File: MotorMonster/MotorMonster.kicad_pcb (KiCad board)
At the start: 4 copper layers, 100 x 100 mm, 83 parts, among them J1 USB C Connector, J3 HV In, SW1 Boot, U1 XC6206, U2 USBLC6-2SC6, U3 RP2040, U4 W25Q128JVS, U5 LM5164DDA, Y1 12MHz

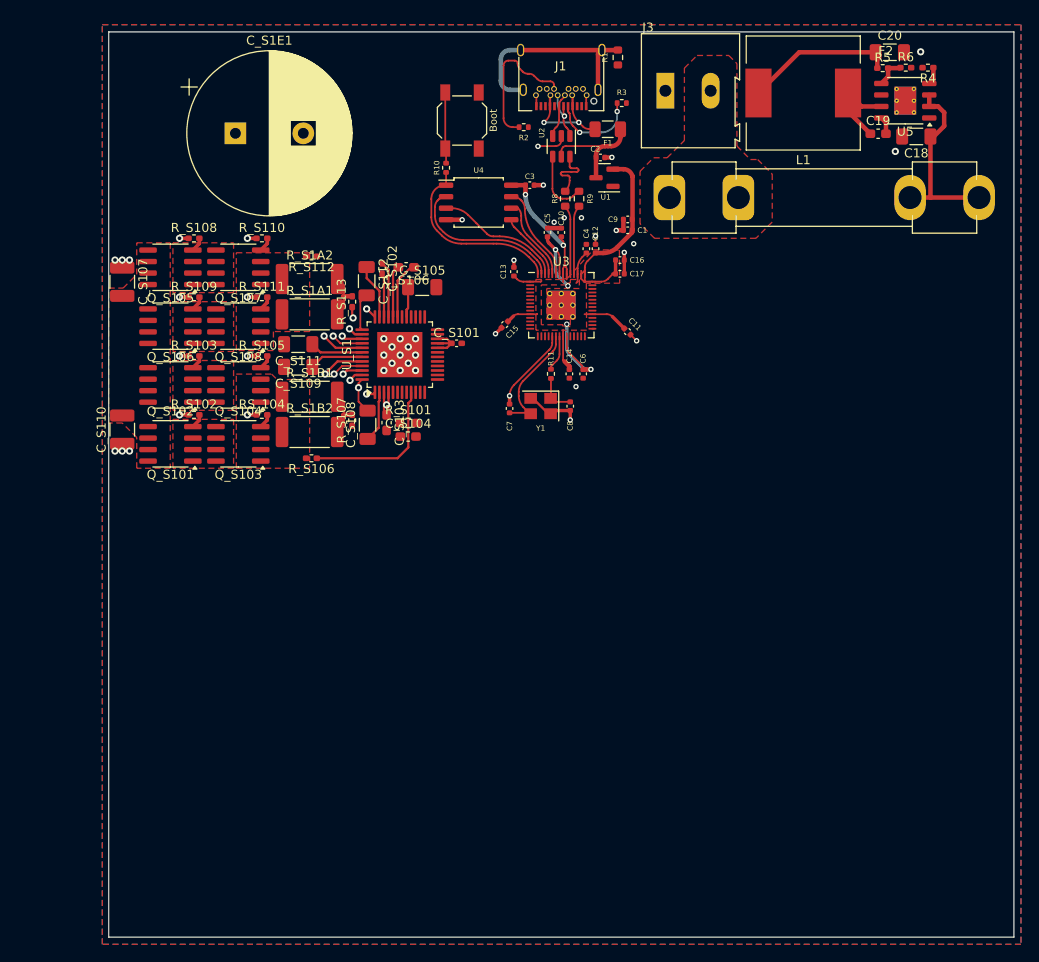
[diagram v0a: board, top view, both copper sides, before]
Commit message: fully laid out
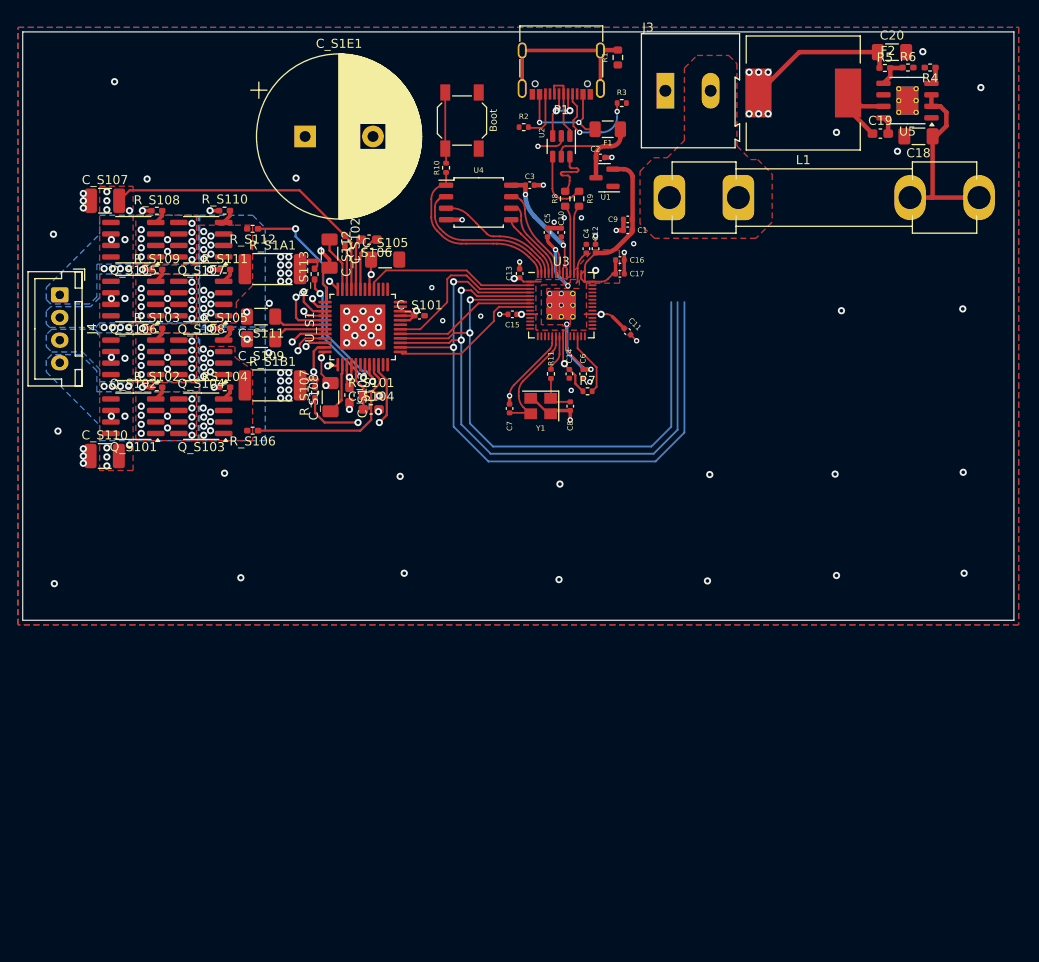
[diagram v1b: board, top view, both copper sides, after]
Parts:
- removed J1: USB C Connector, footprints:TYPE-C_24P_QCHT
- removed R_S1A2, R_S1B2: R, Resistor_SMD:R_2512_6332Metric_Pad1.40x3.35mm_HandSolder
- added J4: Conn_01x04, Connector_JST:JST_XH_B4B-XH-A_1x04_P2.50mm_Vertical, F.Cu at (84.6, 49.0)
- added P1: USB_C_Plug_USB2.0, Connector_USB:USB_C_Receptacle_G-Switch_GT-USB-7010ASV, F.Cu at (140.0, 23.1)
- added R7: 10k, Resistor_SMD:R_0402_1005Metric, F.Cu at (142.9, 59.7)
- moved C_S107 9.15 mm to (89.6, 38.6), turned to 0 degrees
- moved C_S1E1 7.71 mm to (111.7, 31.6)
- moved R_S112 7.18 mm to (105.9, 41.8)
- moved R_S106 7.18 mm to (105.9, 64.0)
- moved R_S1A1 6.47 mm to (108.1, 46.2)
- moved NT1 5.52 mm to (112.5, 58.4)
- moved NT2 5.48 mm to (112.5, 45.3)
- moved R_S113 5.15 mm to (112.8, 46.8)
- moved R_S110 5.14 mm to (102.8, 39.8)
- moved C_S105 5.11 mm to (120.5, 45.1)
- moved Q_S105 5.11 mm to (92.7, 43.0)
- moved Q_S106 5.11 mm to (92.7, 49.5)
- moved Q_S107 5.11 mm to (100.2, 43.0)
- moved Q_S108 5.11 mm to (100.2, 49.5)
- moved C_S101 5.11 mm to (124.3, 51.4)
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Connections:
- U3 pad 2: unconnected-(U3-GPIO0-Pad2) -> S1En
- U3 pad 3: unconnected-(U3-GPIO1-Pad3) -> S1Dir
- U3 pad 7: S1CS -> S1Step
- U3 pad 8: unconnected-(U3-GPIO6-Pad8) -> S1CS
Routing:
- net SPI_CLK: track 0.00 -> 73.7 mm, vias 0 -> 2
- net SPI_DRV_IN: track 0.00 -> 70.0 mm, vias 0 -> 2
- net SPI_DRV_OUT: track 0.00 -> 66.2 mm, vias 0 -> 2
- net Vdrive: track 27.3 -> 54.8 mm, vias 0 -> 28
- net Net-(U_S1-HA2): track 2.28 -> 29.5 mm
- net Net-(U_S1-SRAH): track 0.00 -> 27.2 mm, vias 0 -> 2
- net Net-(U_S1-HA1): track 5.76 -> 30.7 mm
- net Net-(U_S1-HB1): track 1.99 -> 24.2 mm
- net 1A+: track 3.53 -> 23.7 mm, vias 1 -> 13
- net S1En: track 0.00 -> 19.2 mm
- net S1Dir: track 0.00 -> 18.9 mm
- net Net-(U_S1-LA1): track 3.33 -> 21.8 mm
- net 1A-: track 4.17 -> 22.3 mm, vias 0 -> 12
- net S1CS: track 0.00 -> 17.2 mm
- net Net-(U_S1-HB2): track 5.69 -> 22.7 mm
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- added copper zone on In1.Cu, net +12V
- added copper zone on In1.Cu, net +3V3
- added copper zone on B.Cu, net 1A+
- added copper zone on In1.Cu, net 1A+
- added copper zone on B.Cu, net 1A-
- added copper zone on In1.Cu, net 1A-
- added copper zone on B.Cu, net 1B+
- added copper zone on B.Cu, net 1B-
- added copper zone on In1.Cu, net 1B-
- added copper zone on In1.Cu, net GND
- added copper zone on In2.Cu, net GND
- added copper zone on B.Cu, net S1A_Ret
- added copper zone on B.Cu, net S1B_Ret
- added copper zone on In1.Cu, net Vdrive
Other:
- board size 100 x 100 mm -> 109.5 x 65 mm
